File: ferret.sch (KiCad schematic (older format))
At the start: 55 parts

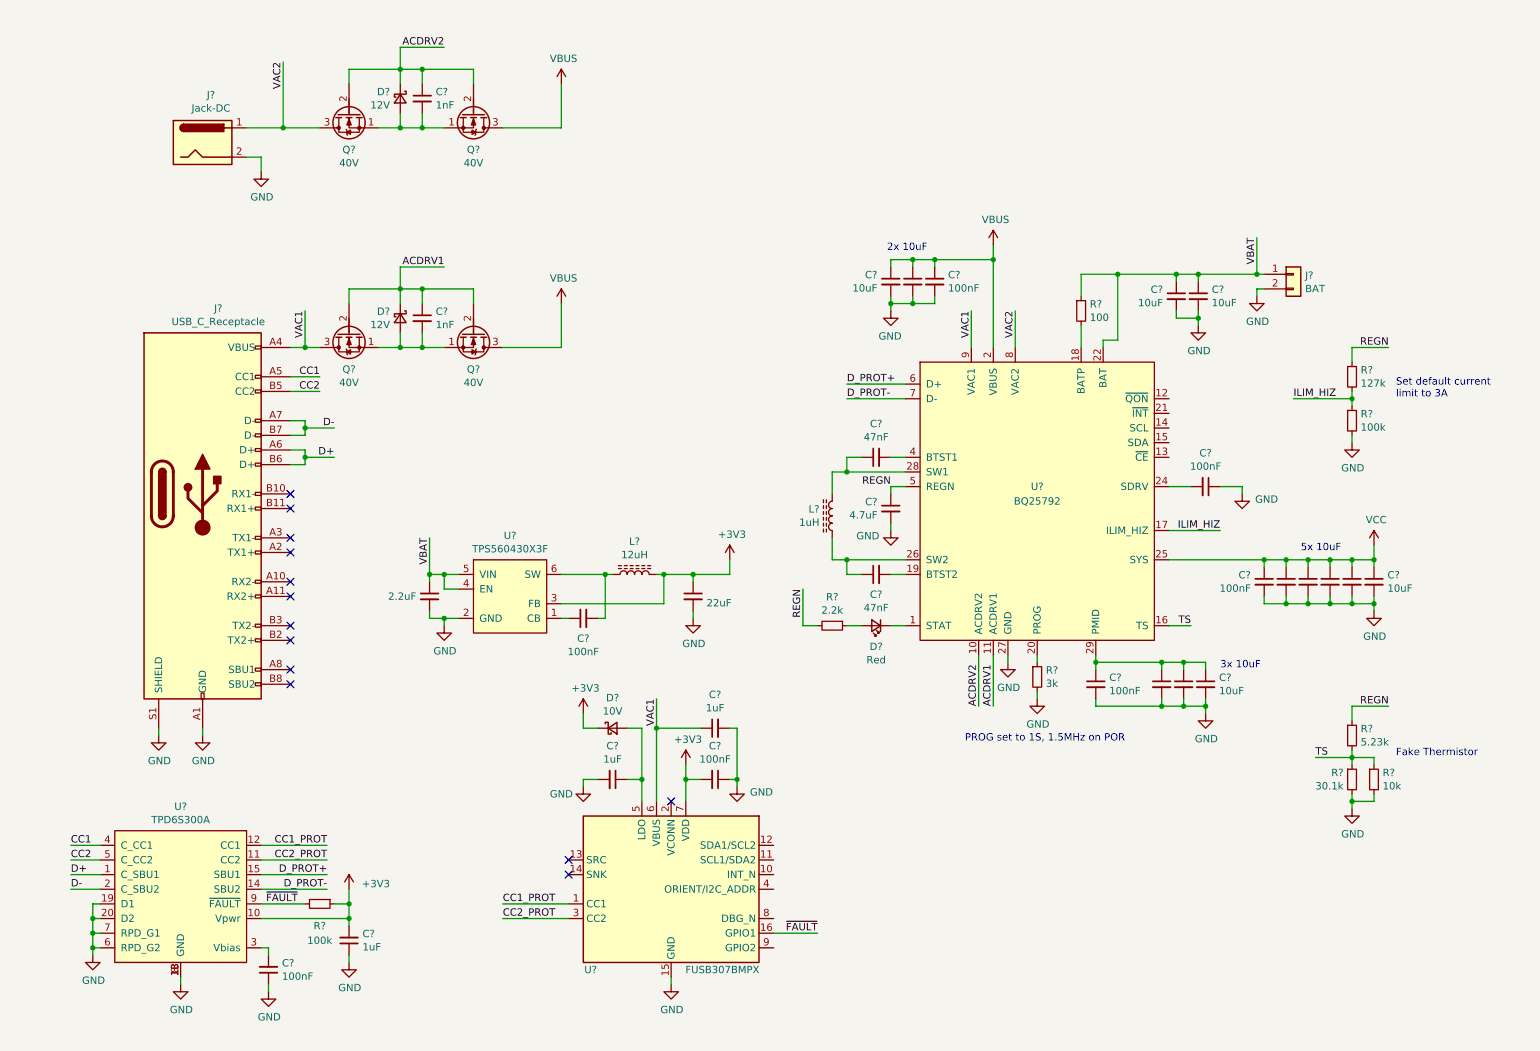
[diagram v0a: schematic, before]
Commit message: Schematic is pretty much finished now
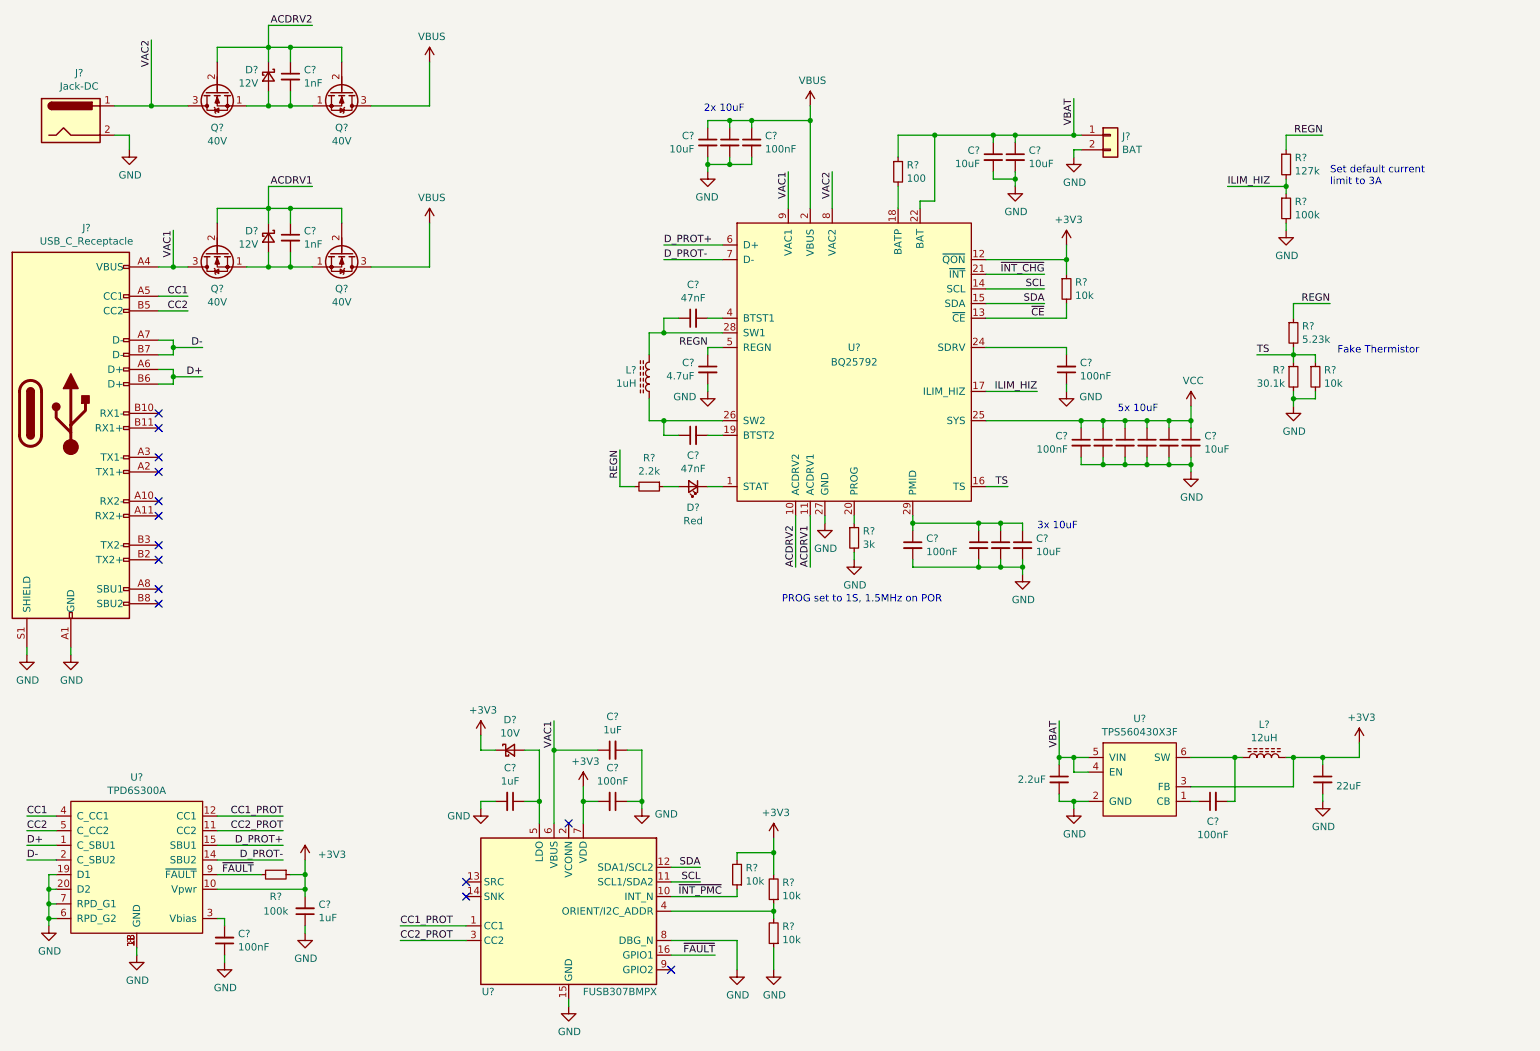
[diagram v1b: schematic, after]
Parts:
- added R? (x4): 10k, Resistor_SMD:R_0603_1608Metric, symbol Device:R_Small
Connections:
- net +3V3: now also U?.12 (~QON), R?.1, R?.2, R?.2
- net GND: now also U?.8 (DBG_N), R?.1
- net ~CE: now reaches U?.13 (~CE)
- net ~CE: now also R?.2
- net SCL: now reaches U?.14 (SCL)
- net SCL: now also U?.11 (SCL1/SDA2)
- net SDA: now reaches U?.15 (SDA)
- net SDA: now also U?.12 (SDA1/SCL2)
- net ~INT_CHG: now reaches U?.21 (~INT)
- net ~INT_PMC: now reaches U?.10 (INT_N)
- net ~INT_PMC: now also R?.1
- net at U?.4 (ORIENT/I2C_ADDR): now also R?.1, R?.2
- no-connect marks 13 -> 14
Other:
- moved on the sheet: C?, D?, J?, L?, Q?, R?, U?

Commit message: some shuffeling
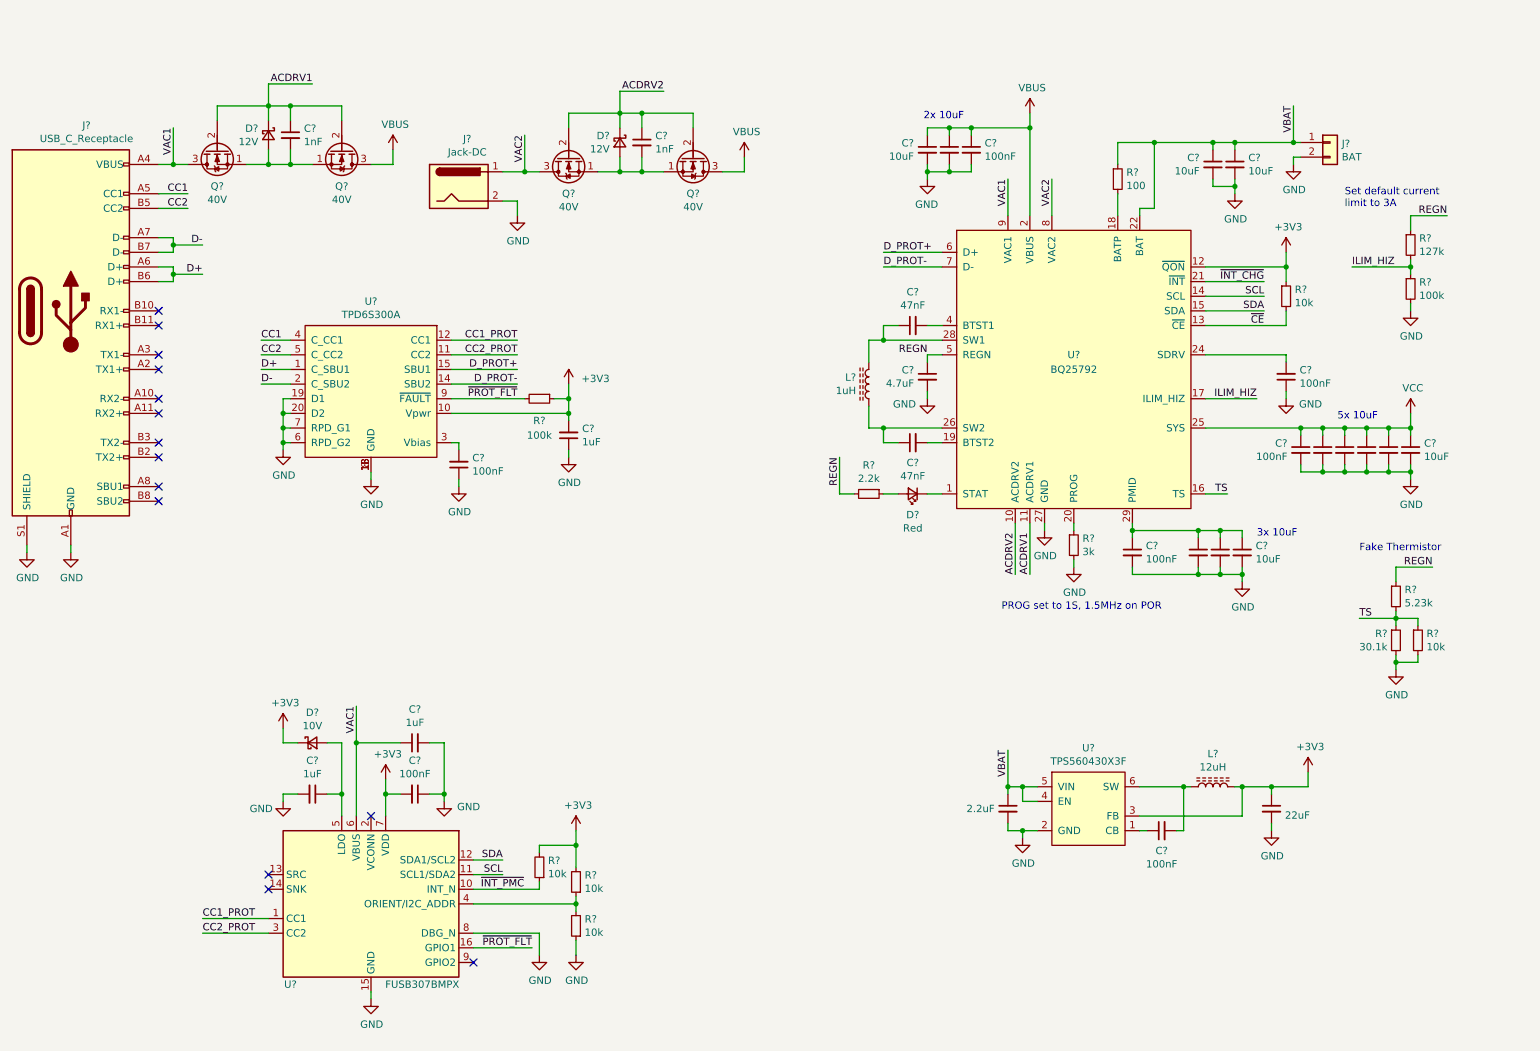
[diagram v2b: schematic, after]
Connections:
- net ~FAULT renamed ~PROT_FLT
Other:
- moved on the sheet: C?, D?, J?, L?, Q?, R?, U?
